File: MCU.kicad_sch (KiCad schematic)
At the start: 20 parts, among them J3 ADC_EXT_SUPPLY, J4 MCU_V_SEL, U2 LPC55S28JBD100

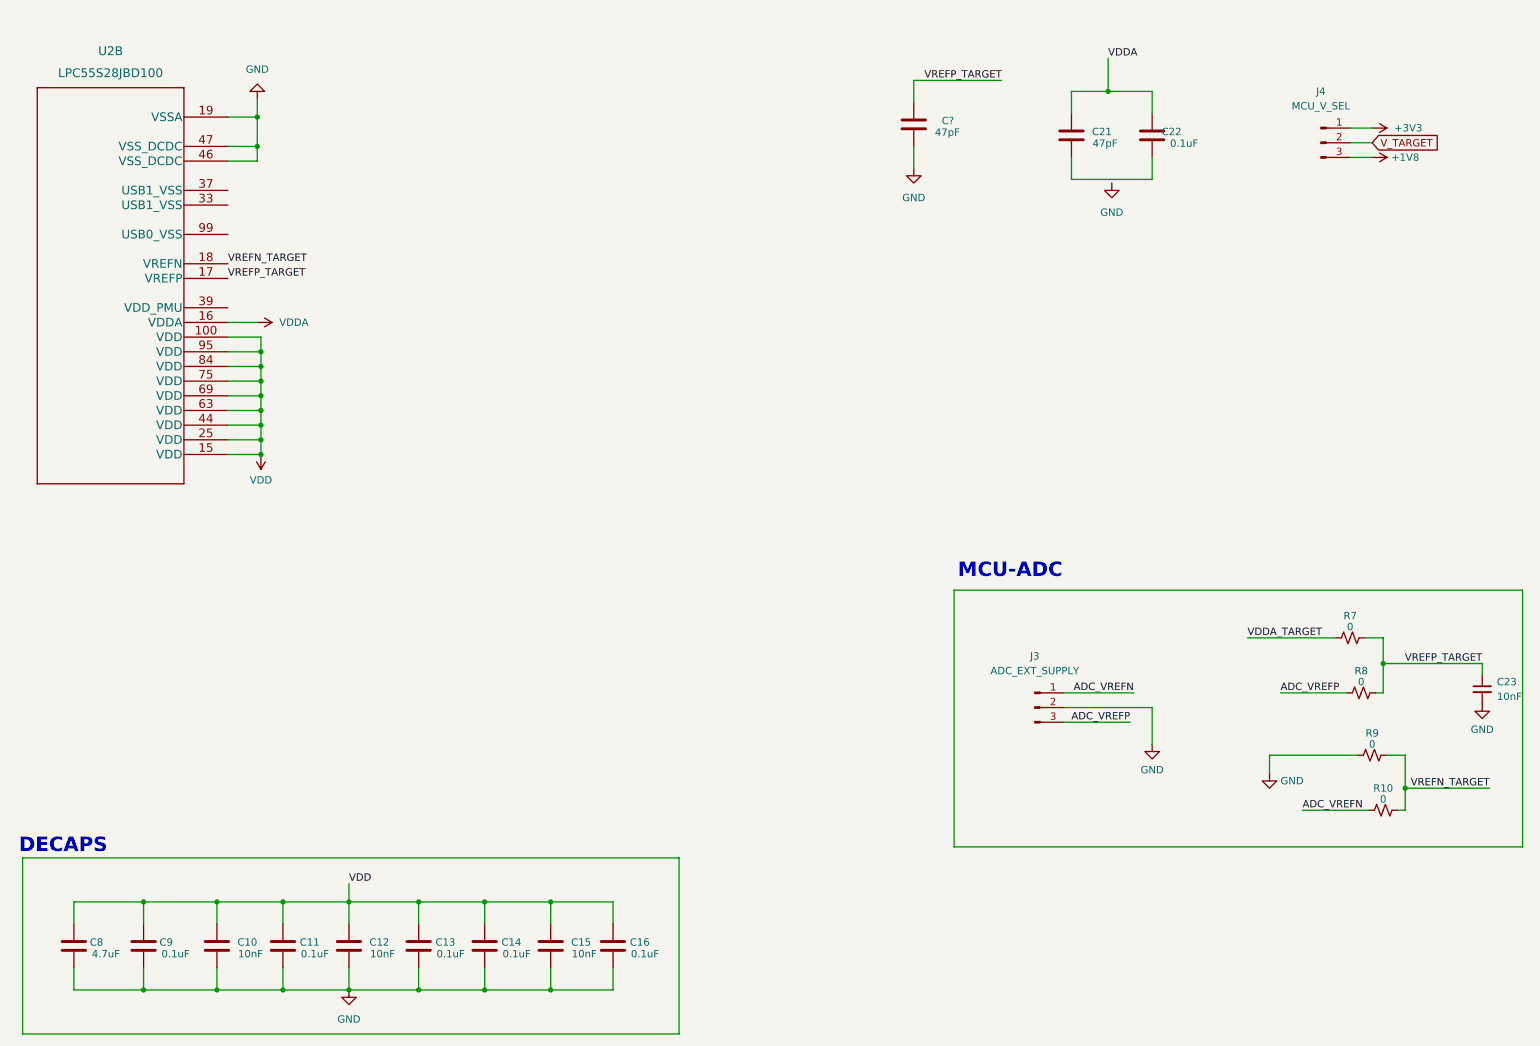
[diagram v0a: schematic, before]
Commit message: Reset devresi eklenecek.
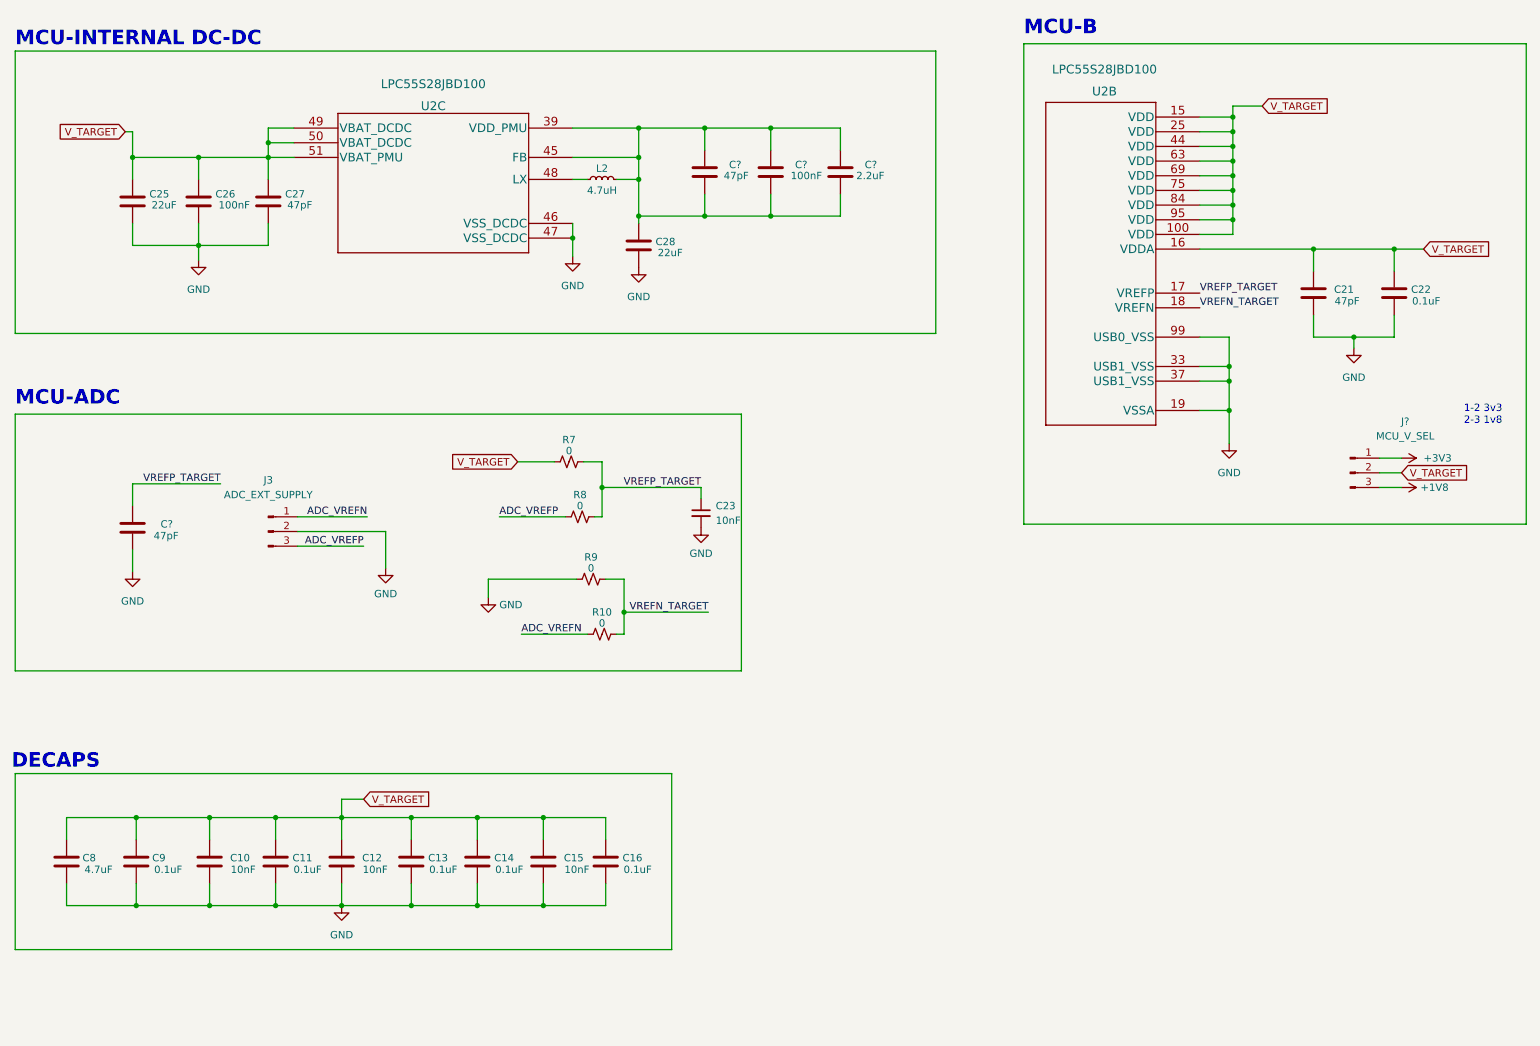
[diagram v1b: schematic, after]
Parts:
- removed C?: 47pF, Resistor_SMD:R_0603_1608Metric, symbol Device:C
- removed J4: MCU_V_SEL, Connector_PinHeader_2.54mm:PinHeader_1x03_P2.54mm_Vertical, symbol Connector:Conn_01x03_Male
- added C25, C28: 22uF, Resistor_SMD:R_0603_1608Metric, symbol Device:C
- added C26, C?: 100nF, Resistor_SMD:R_0603_1608Metric, symbol Device:C
- added C27, C? (x2): 47pF, Resistor_SMD:R_0603_1608Metric, symbol Device:C
- added C?: 2.2uF, Resistor_SMD:R_0603_1608Metric, symbol Device:C
- added J?: MCU_V_SEL, Connector_PinHeader_2.54mm:PinHeader_1x03_P2.54mm_Vertical, symbol Connector:Conn_01x03_Male
- added L2: 4.7uH, symbol Device:L_Small
- added unit 3 of U2
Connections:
- net VDD is gone; now on net V_TARGET: C10.1, C11.1, C12.1, C13.1, C14.1, C15.1, C16.1, C8.1, C9.1, U2.100 (VDD), U2.15 (VDD), U2.25 (VDD), U2.44 (VDD), U2.63 (VDD), U2.69 (VDD), U2.75 (VDD), U2.84 (VDD), U2.95 (VDD)
- net VDDA is gone; now on net V_TARGET: C21.1, C22.1, U2.16 (VDDA)
- net VDDA_TARGET is gone; now on net V_TARGET: R7.1
- net +1V8: now also J?.3 (Pin_3)
- net +3V3: now also J?.1 (Pin_1)
- net GND: now also C21.2, C22.2, U2.33 (USB1_VSS), U2.37 (USB1_VSS), U2.99 (USB0_VSS), C25.2, C26.2, C27.2, C28.2, C?.2, U2.46 (VSS_DCDC), U2.47 (VSS_DCDC); no longer U2.46 (VSS_DCDC), U2.47 (VSS_DCDC)
- net VREFP_TARGET: now also C?.1
- net V_TARGET: now also C25.1, C26.1, C27.1, J?.2 (Pin_2), U2.49 (VBAT_DCDC), U2.50 (VBAT_DCDC), U2.51 (VBAT_PMU)
- new net: C28.1, C?.1, C?.1, C?.1, C?.2, C?.2, C?.2, L2.2, U2.39 (VDD_PMU), U2.45 (FB)
- new net: L2.1, U2.48 (LX)
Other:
- note added: "1-2 3v3 2-3 1v8"
- note added: "MCU-B"
- note added: "MCU-INTERNAL DC-DC"
- moved on the sheet: C10, C11, C12, C13, C14, C15, C16, C23, C8, C9, J3, R10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
